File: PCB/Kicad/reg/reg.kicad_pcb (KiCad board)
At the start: 6 copper layers, 200 x 150 mm, 226 parts, among them J4 Conn_02x10_Odd_Even, J5 Conn_02x10_Odd_Even, J6 Conn_02x10_Odd_Even, U1 74377, U10 74245, U107 74245, U108 74245, U109 74245, U11 74245, U110 74245, U111 74245, U112 74245, U113 74245, U114 74245, U115 74245, U116 74245, U117 74245, U118 74245, U119 74245, U12 74245, U120 74245, U121 74245, U122 74245, U123 74245, U124 74245, U125 74245, U126 74245, U127 74245, U128 74245, U129 74245, U130 74245, U131 74245, U132 74245, U133 74245, U134 74245, U135 74245, U136 74245, U14 74377, U15 74245, U16 74245, U17 7404, U18 74377, U19 74377, U2 7400, U20 74377, U21 74245, U22 74245, U23 74377, U24 74377, U25 74377, U26 74377, U27 74377, U28 74377, U29 744067, U3 7400, U30 744067, U31 74377, U32 74377, U33 74377, U34 74377, U35 74377, U36 74377, U37 74377, U38 74377, U39 74377, U4 7400, U40 74377, U41 74377, U42 74377, U43 74377, U44 74377, U45 74377, U46 74377, U47 74377, U48 74377, U49 74377, U5 74245, U50 74377, U51 74377, U52 74377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

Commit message: routes
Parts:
- moved U92 122.4 mm to (97.8, 143.2)
- moved U91 120.7 mm to (109.5, 143.2)
- moved U82 100.8 mm to (185.0, 62.4)
- moved U51 100.8 mm to (173.2, 61.8)
- moved U120 99.3 mm to (139.6, 75.7)
- moved U27 99.3 mm to (127.9, 75.2)
- moved U135 97.5 mm to (163.2, 62.8)
- moved U52 97.5 mm to (151.0, 62.6)
- moved U53 97.4 mm to (128.3, 158.9)
- moved U81 97.4 mm to (140.0, 159.5)
- moved U2 97.0 mm to (36.6, 45.6), turned to -90 degrees
- moved U3 91.6 mm to (50.0, 43.2)
- moved U125 89.6 mm to (209.6, 129.3)
- moved U41 89.6 mm to (198.1, 128.8)
- moved U123 82.5 mm to (209.8, 144.7)
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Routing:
- net /data15: track 0.00 -> 242.9 mm, vias 0 -> 18
- net /data8: track 0.00 -> 242.8 mm, vias 0 -> 18
- net /data14: track 0.00 -> 242.6 mm, vias 0 -> 18
- net /data9: track 0.00 -> 242.1 mm, vias 0 -> 18
- net /data10: track 0.00 -> 240.9 mm, vias 0 -> 18
- net /data13: track 0.00 -> 239.0 mm, vias 0 -> 18
- net /data11: track 0.00 -> 238.6 mm, vias 0 -> 18
- net /data12: track 0.00 -> 237.7 mm, vias 0 -> 18
- net /OUT_1_8: track 8.11 -> 149.7 mm, vias 0 -> 3
- net /OUT_7_7: track 7.92 -> 141.8 mm, vias 1 -> 3
- net /OUT_7_8: track 7.18 -> 139.7 mm, vias 1 -> 2
- net /OUT_1_9: track 7.47 -> 131.1 mm, vias 0 -> 3
- net /OUT_7_9: track 6.44 -> 123.0 mm, vias 1 -> 2
- net /OUT_7_6: track 7.36 -> 123.5 mm, vias 1 -> 3
- net /OUT_1_10: track 6.91 -> 116.5 mm, vias 0 -> 3
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
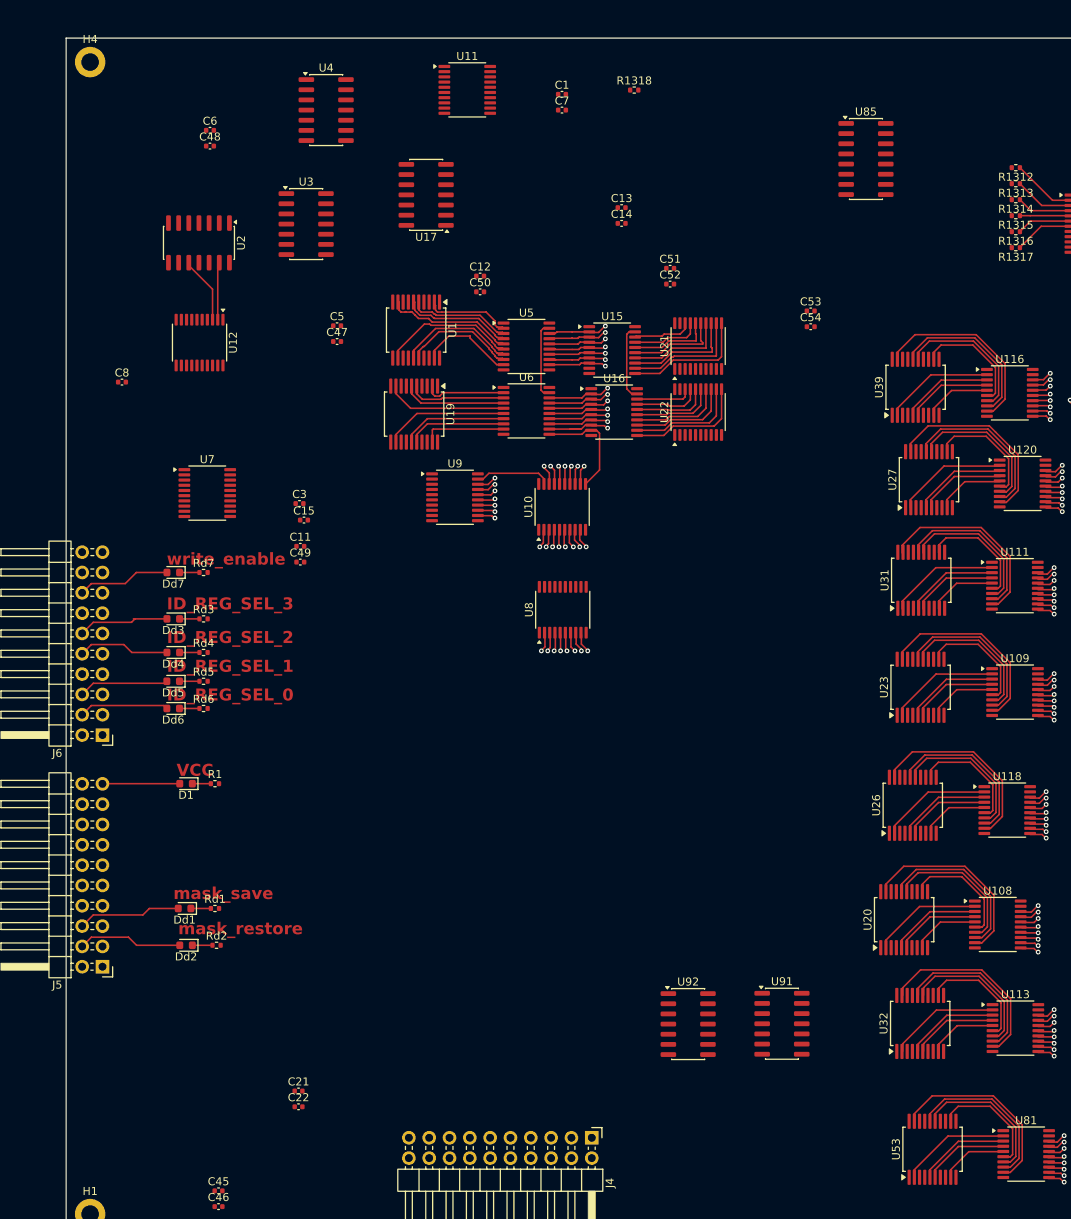
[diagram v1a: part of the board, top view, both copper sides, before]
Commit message: mess
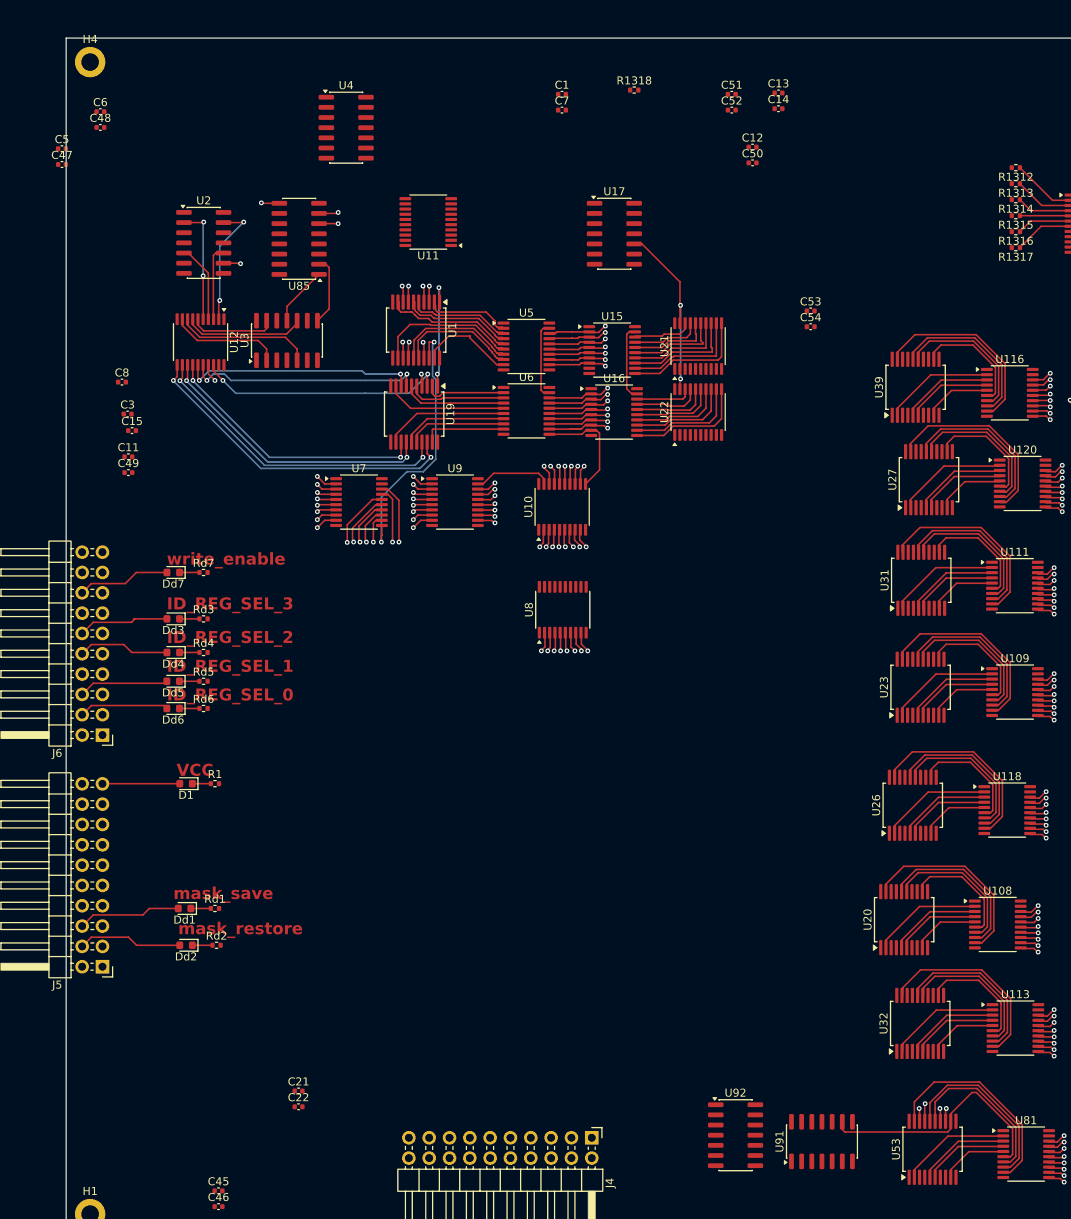
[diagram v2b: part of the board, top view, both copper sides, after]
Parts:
- moved U85 71.5 mm to (49.1, 45.1), turned to 180 degrees
- moved C47 40.9 mm to (19.5, 35.8)
- moved C5 40.9 mm to (19.5, 33.8)
- moved C12 37.7 mm to (105.8, 33.6)
- moved C50 37.7 mm to (105.8, 35.6)
- moved C13 24.3 mm to (109.0, 26.9)
- moved C14 24.3 mm to (109.0, 28.8)
- moved C11 24.2 mm to (27.8, 72.3)
- moved C3 24.2 mm to (27.7, 67.0)
- moved C49 24.2 mm to (27.8, 74.3)
- moved C15 24.2 mm to (28.2, 69.1)
- moved U17 24.0 mm to (88.5, 44.5), turned to 0 degrees
- moved C51 23.1 mm to (103.2, 27.0)
- moved C52 23.1 mm to (103.2, 29.0)
- moved U7 19.0 mm to (56.6, 78.0)
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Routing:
- net /data0: track 27.7 -> 117.5 mm, vias 12 -> 14
- net /data1: track 27.5 -> 113.2 mm, vias 12 -> 14
- net /data2: track 26.8 -> 108.3 mm, vias 12 -> 14
- net /data3: track 25.0 -> 102.7 mm, vias 12 -> 14
- net /data4: track 24.3 -> 98.3 mm, vias 12 -> 14
- net /data5: track 25.0 -> 95.5 mm, vias 12 -> 14
- net /data6: track 25.8 -> 92.7 mm, vias 12 -> 14
- net /data7: track 26.5 -> 89.7 mm, vias 12 -> 14
- net /16 bit buffor23/OUT2: track 0.00 -> 46.7 mm, vias 0 -> 2
- net /16 bit buffor23/OUT0: track 0.00 -> 43.5 mm, vias 0 -> 2
- net /16 bit buffor23/OUT3: track 0.00 -> 43.2 mm, vias 0 -> 2
- net /16 bit buffor23/OUT1: track 0.00 -> 42.6 mm, vias 0 -> 2
- net /16 bit buffor23/OUT15: track 0.00 -> 41.6 mm, vias 0 -> 2
- net /16 bit buffor23/OUT14: track 0.00 -> 39.2 mm, vias 0 -> 2
- net /16 bit buffor23/OUT13: track 0.00 -> 36.0 mm, vias 0 -> 2
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
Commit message: routes
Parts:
- moved U135 486.9 mm to (649.8, 80.3)
- moved U52 486.9 mm to (637.6, 80.1)
- moved U132 458.1 mm to (621.2, 92.3)
- moved U47 458.1 mm to (609.1, 92.1)
- moved U48 442.0 mm to (637.7, 92.1)
- moved U136 442.0 mm to (649.5, 92.6)
- moved U133 427.4 mm to (590.3, 76.8)
- moved U49 427.4 mm to (578.6, 76.4)
- moved U131 412.7 mm to (621.5, 80.0)
- moved U50 412.7 mm to (609.6, 79.4)
- moved U130 397.8 mm to (560.8, 91.4)
- moved U43 397.8 mm to (549.0, 91.1)
- moved U134 381.0 mm to (590.0, 91.7)
- moved U44 381.0 mm to (578.3, 91.3)
- moved U127 365.8 mm to (527.1, 74.4)
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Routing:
- net /data7: track 89.7 -> 483.0 mm, vias 14 -> 24
- net /data6: track 92.7 -> 456.6 mm, vias 14 -> 24
- net /data5: track 95.5 -> 424.4 mm, vias 14 -> 24
- net /data4: track 98.3 -> 396.8 mm, vias 14 -> 24
- net /data3: track 102.7 -> 381.9 mm, vias 14 -> 27
- net /data1: track 113.2 -> 389.8 mm, vias 14 -> 27
- net /data2: track 108.3 -> 378.1 mm, vias 14 -> 27
- net /data0: track 117.5 -> 385.0 mm, vias 14 -> 27
- net /data15: track 242.9 -> 478.5 mm, vias 18 -> 24
- net /data14: track 242.6 -> 472.0 mm, vias 18 -> 24
- net /data13: track 239.0 -> 418.5 mm, vias 18 -> 24
- net /data12: track 237.7 -> 404.7 mm, vias 18 -> 24
- net /data9: track 242.1 -> 385.7 mm, vias 18 -> 24
- net /OUT_1_8: track 149.7 -> 8.11 mm, vias 3 -> 1
- net /data11: track 238.6 -> 378.9 mm, vias 18 -> 24
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
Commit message: spaghetti
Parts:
- moved U135 445.6 mm to (207.0, 30.3)
- moved U136 445.1 mm to (207.1, 43.4)
- moved U52 445.0 mm to (195.4, 29.6)
- moved U48 444.9 mm to (195.6, 42.7)
- moved U132 444.0 mm to (179.9, 43.4)
- moved U131 443.7 mm to (180.6, 30.3)
- moved U47 443.6 mm to (168.3, 42.8)
- moved U50 443.5 mm to (168.9, 29.7)
- moved U49 441.4 mm to (139.7, 29.7)
- moved U133 441.3 mm to (151.4, 30.4)
- moved U134 441.1 mm to (151.6, 43.4)
- moved U44 441.1 mm to (139.9, 42.7)
- moved U43 438.0 mm to (113.8, 42.7)
- moved U46 437.9 mm to (113.8, 29.7)
- moved U130 437.9 mm to (125.5, 43.4)
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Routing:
- net /clk: track 0.00 -> 1121.1 mm, vias 0 -> 35
- net /data7: track 483.0 -> 1063.1 mm, vias 24 -> 33
- net /data15: track 478.5 -> 1055.7 mm, vias 24 -> 32
- net /data6: track 456.6 -> 1021.4 mm, vias 24 -> 33
- net /data14: track 472.0 -> 1036.4 mm, vias 24 -> 32
- net /data8: track 370.9 -> 928.0 mm, vias 24 -> 32
- net /data9: track 385.7 -> 936.0 mm, vias 24 -> 32
- net /data13: track 418.5 -> 966.2 mm, vias 24 -> 32
- net /data5: track 424.4 -> 970.7 mm, vias 24 -> 33
- net /data1: track 389.8 -> 926.9 mm, vias 27 -> 33
- net /data10: track 366.1 -> 903.0 mm, vias 24 -> 32
- net /data12: track 404.7 -> 939.8 mm, vias 24 -> 32
- net /data0: track 385.0 -> 919.5 mm, vias 27 -> 33
- net /data11: track 378.9 -> 911.2 mm, vias 24 -> 32
- net /data4: track 396.8 -> 928.8 mm, vias 24 -> 33
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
